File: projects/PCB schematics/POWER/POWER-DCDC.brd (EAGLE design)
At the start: 99.1 x 99.1 mm, 15 parts, among them J3 2P_1-770166-0, J4 2P_1-770166-0, X1 5566-2, X2 5566-2, X3 5566-2, X4 5566-2

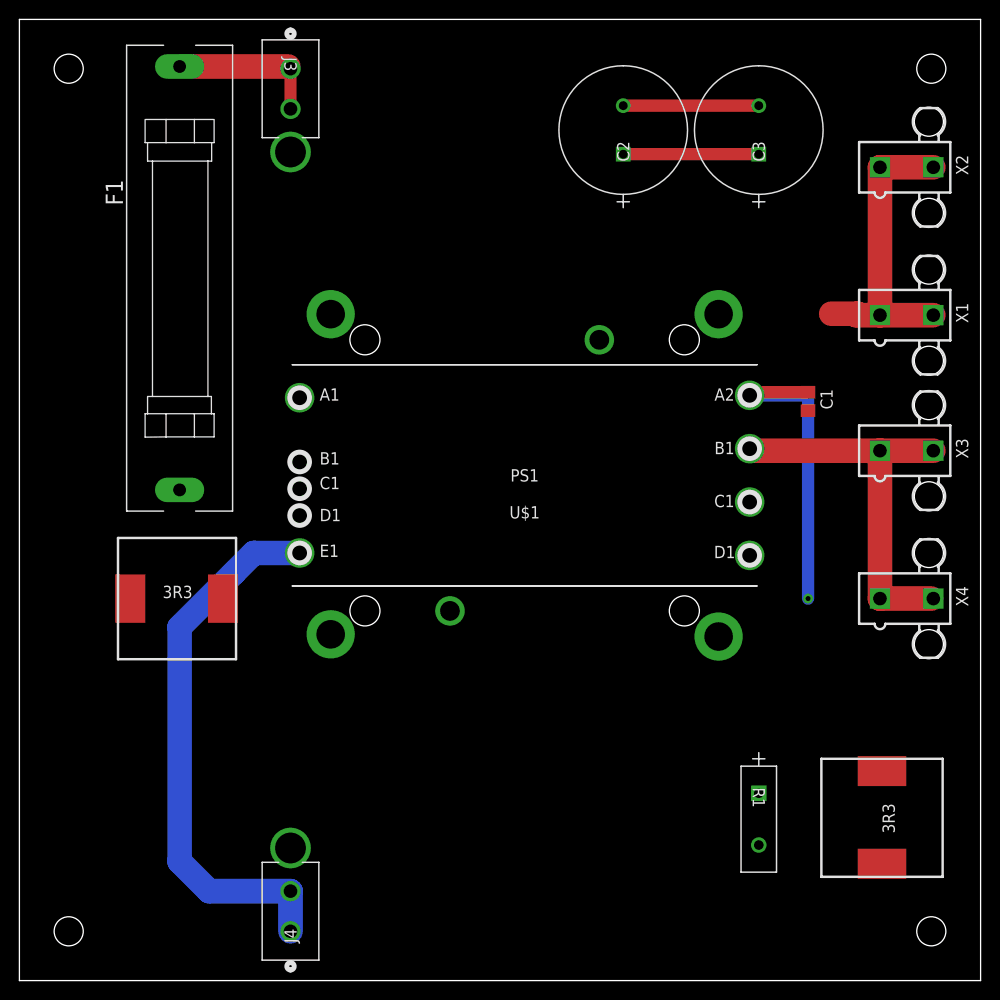
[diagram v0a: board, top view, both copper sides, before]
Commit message: POWER - DCDC Rev A.
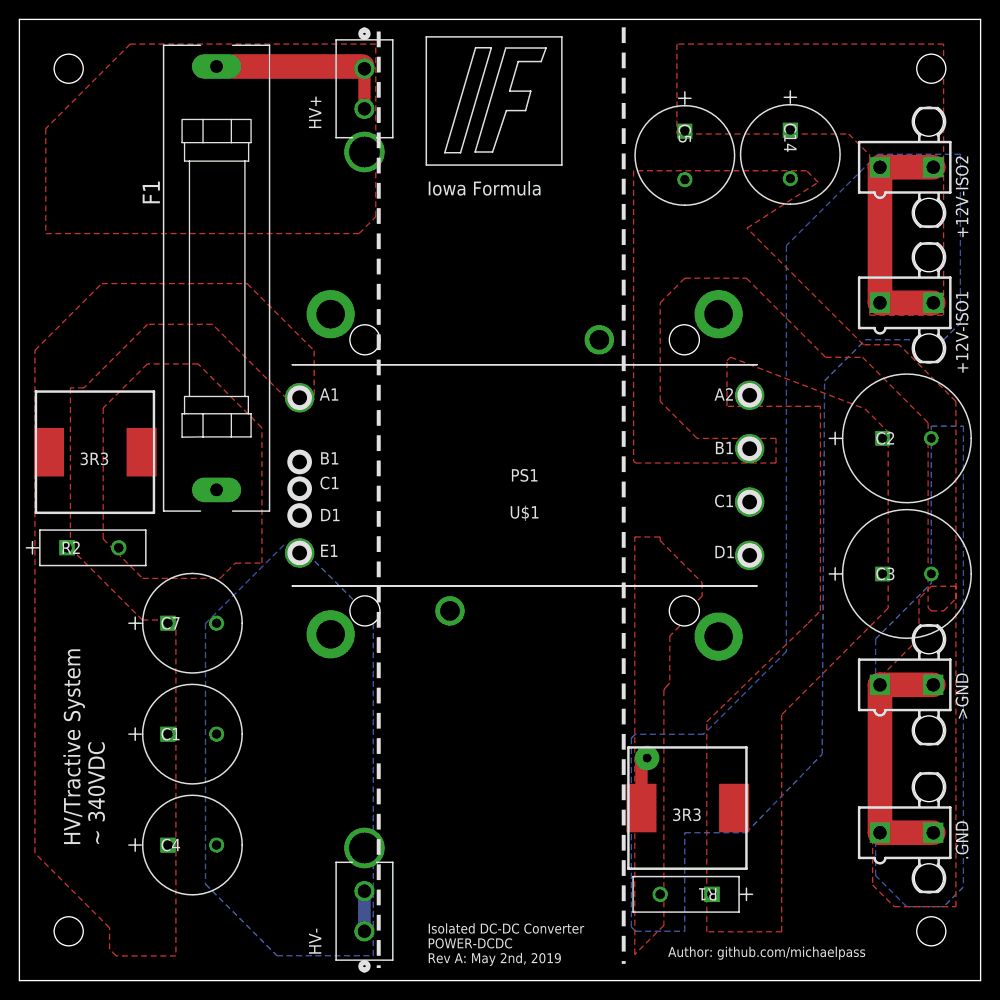
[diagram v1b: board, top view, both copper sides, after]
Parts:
- removed J3, J4: 2P_1-770166-0, con-MATE-N-LOK:CON2_1X2_P163_VMNL-1MTG
- removed U$2: SRP1238A-R22M, IowaFormula:SRP1238A-R22M
- removed X1, X3, X4: 5566-2, con-molex:5566-2
- added +12V-ISO1, .GND, >GND: 5566-2, con-molex:5566-2
- added C14, C4, C5, C7: ECA-2WHG2R2, IowaFormula:PCAP_10X125
- added HV+, HV-: 2P_1-770166-0, con-MATE-N-LOK:CON2_1X2_P163_VMNL-1MTG
- added R2: PWR221T-30-1R00F, IowaFormula:BO_PWR221T
- added U$4: SRP1238A-4R7M, IowaFormula:SRP1238A-R22M
- C1: value 1u -> ECA-2WHG2R2; device rcl:C0805 -> IowaFormula:PCAP_10X125
- moved C1 69.9 mm to (20.3, 25.4), turned to 0 degrees
- moved C3 51.4 mm to (94.0, 41.9), turned to 0 degrees
- moved C2 46.7 mm to (94.0, 55.9), turned to 0 degrees
- moved U$3 15.1 mm to (12.6, 54.5), turned to 180 degrees
- moved R1 11.4 mm to (66.0, 8.89), turned to 180 degrees
- moved F1 3.81 mm to (20.3, 72.4)
- renumbered X2 to +12V-ISO2
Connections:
- removed net HV+_IN: PS1.A1, U$3.2
- net +12V-ISO: now also +12V-ISO1.1, +12V-ISO1.2, C14.1, C5.1, R1.2, U$4.2; no longer X1.1, X1.2
- net +12V-OUT: now also U$4.1; no longer C1.1, U$2.1
- net GND: now also .GND.1, .GND.2, >GND.1, >GND.2, C14.2, C5.2; no longer C1.2, X3.1, X3.2, X4.1, X4.2
- net HV+: now also HV+.1, HV+.2; no longer J3.1, J3.2
- net HV+_POSTFUSE: now also R2.2
- net HV-: now also C1.2, C4.2, C7.2, HV-.1, HV-.2; no longer J4.1, J4.2
- net N$1: now also C1.1, C4.1, C7.1, PS1.A1, R2.1, U$3.2; no longer R1.2, U$2.2
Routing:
- net HV-: track 56.5 -> 4.14 mm
- net +12V-OUT: track 47.1 -> 0.00 mm, vias 1 -> 0
- net GND: track 53.2 -> 26.2 mm
- net HV+: track 15.7 -> 19.5 mm
- net +12V-ISO: track 31.6 -> 30.4 mm, vias 0 -> 1
- added copper zone on layer 1, net +12V-ISO
- added copper zone on layer 16, net +12V-ISO
- added copper zone on layer 1, net +12V-OUT
- added copper zone on layer 1, net GND
- added copper zone on layer 16, net GND
- added copper zone on layer 1, net HV+
- added copper zone on layer 1, net HV+_POSTFUSE
- added copper zone on layer 16, net HV-
- added copper zone on layer 1, net N$1
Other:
- board text added: "Author: github.com/michaelpass"
- board text added: "HV/Tractive System ~ 340VDC"
- board text added: "Iowa Formula"
- board text added: "Isolated DC-DC Converter POWER-DCDC Rev A: May 2nd, 2019"
